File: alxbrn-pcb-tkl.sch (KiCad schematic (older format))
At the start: 24 parts, among them SW1 SW_Push, U1 ATmega32U4-AU, Y1 16MHz

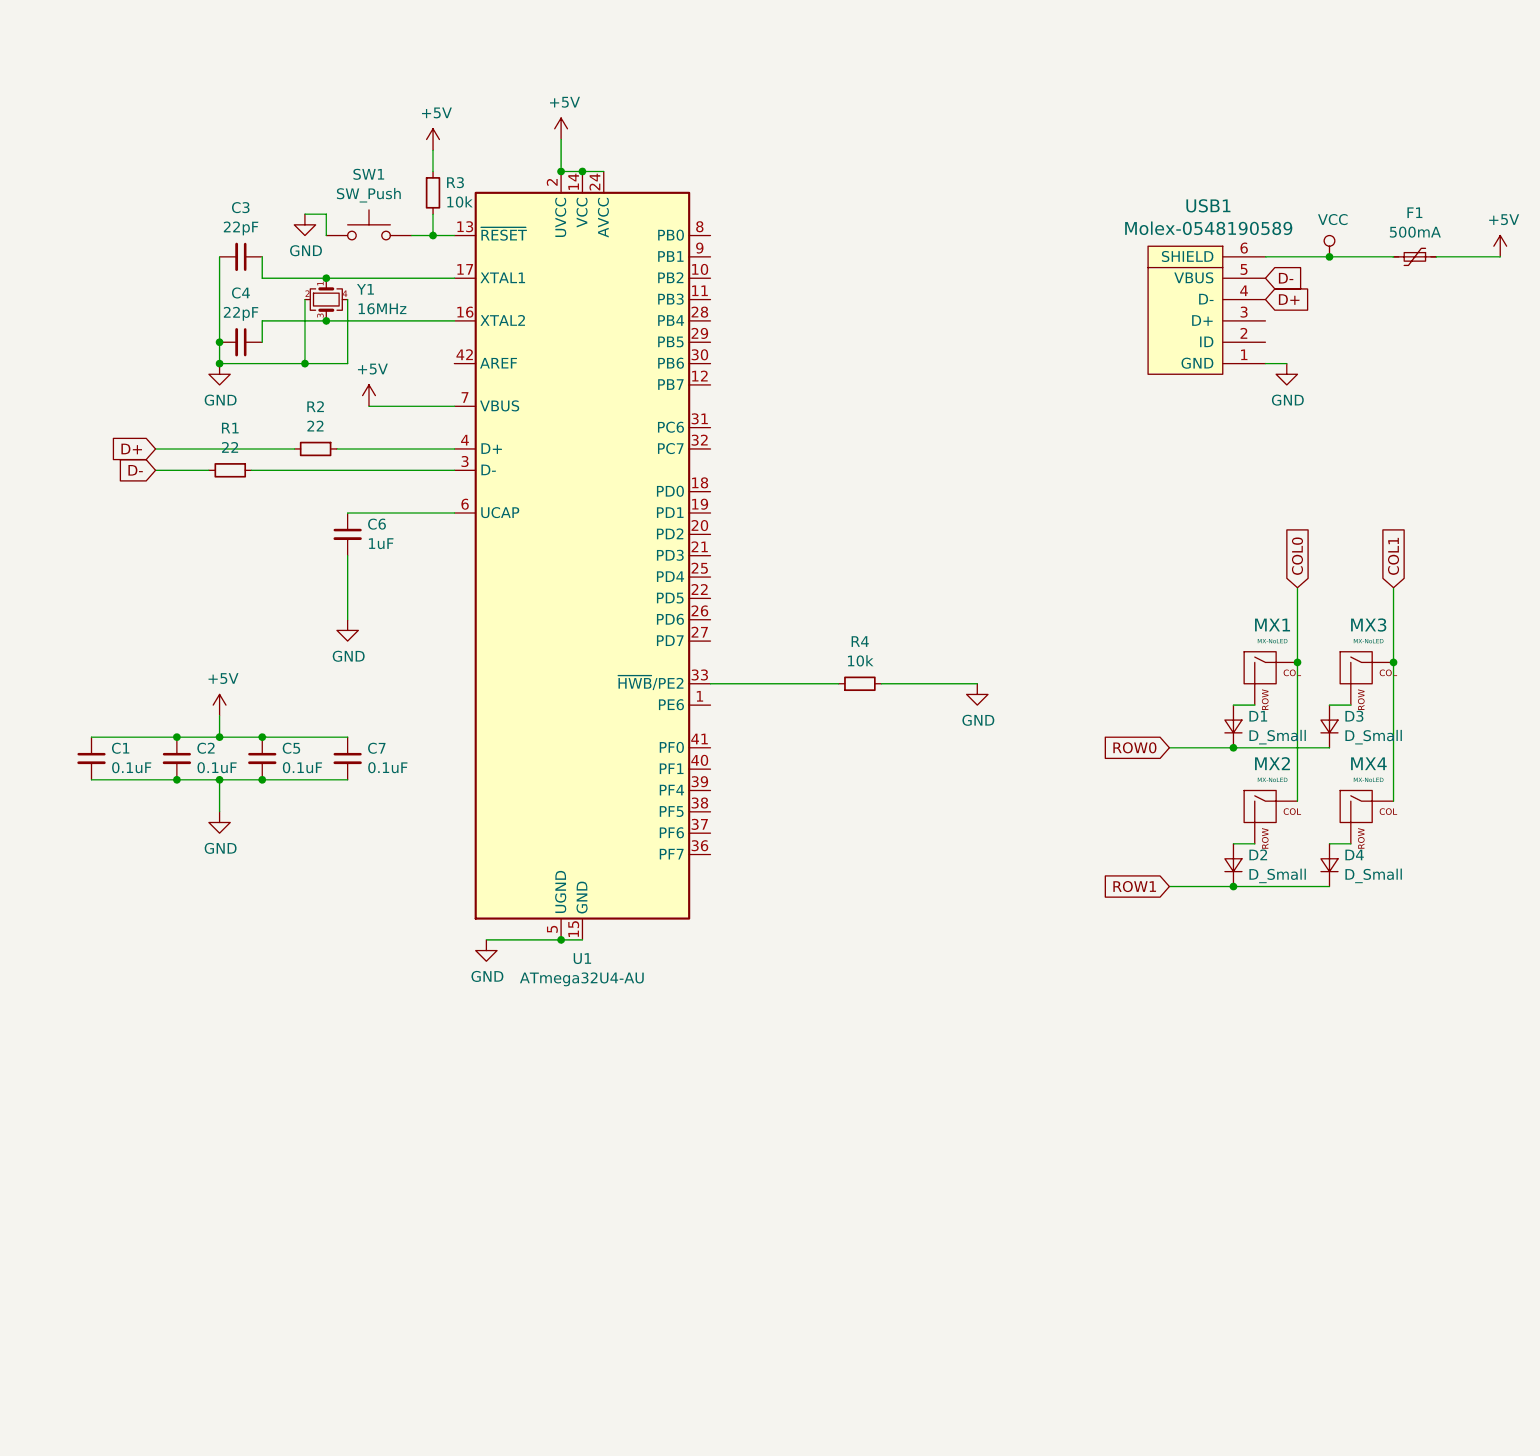
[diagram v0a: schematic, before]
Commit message: Schematic finished.
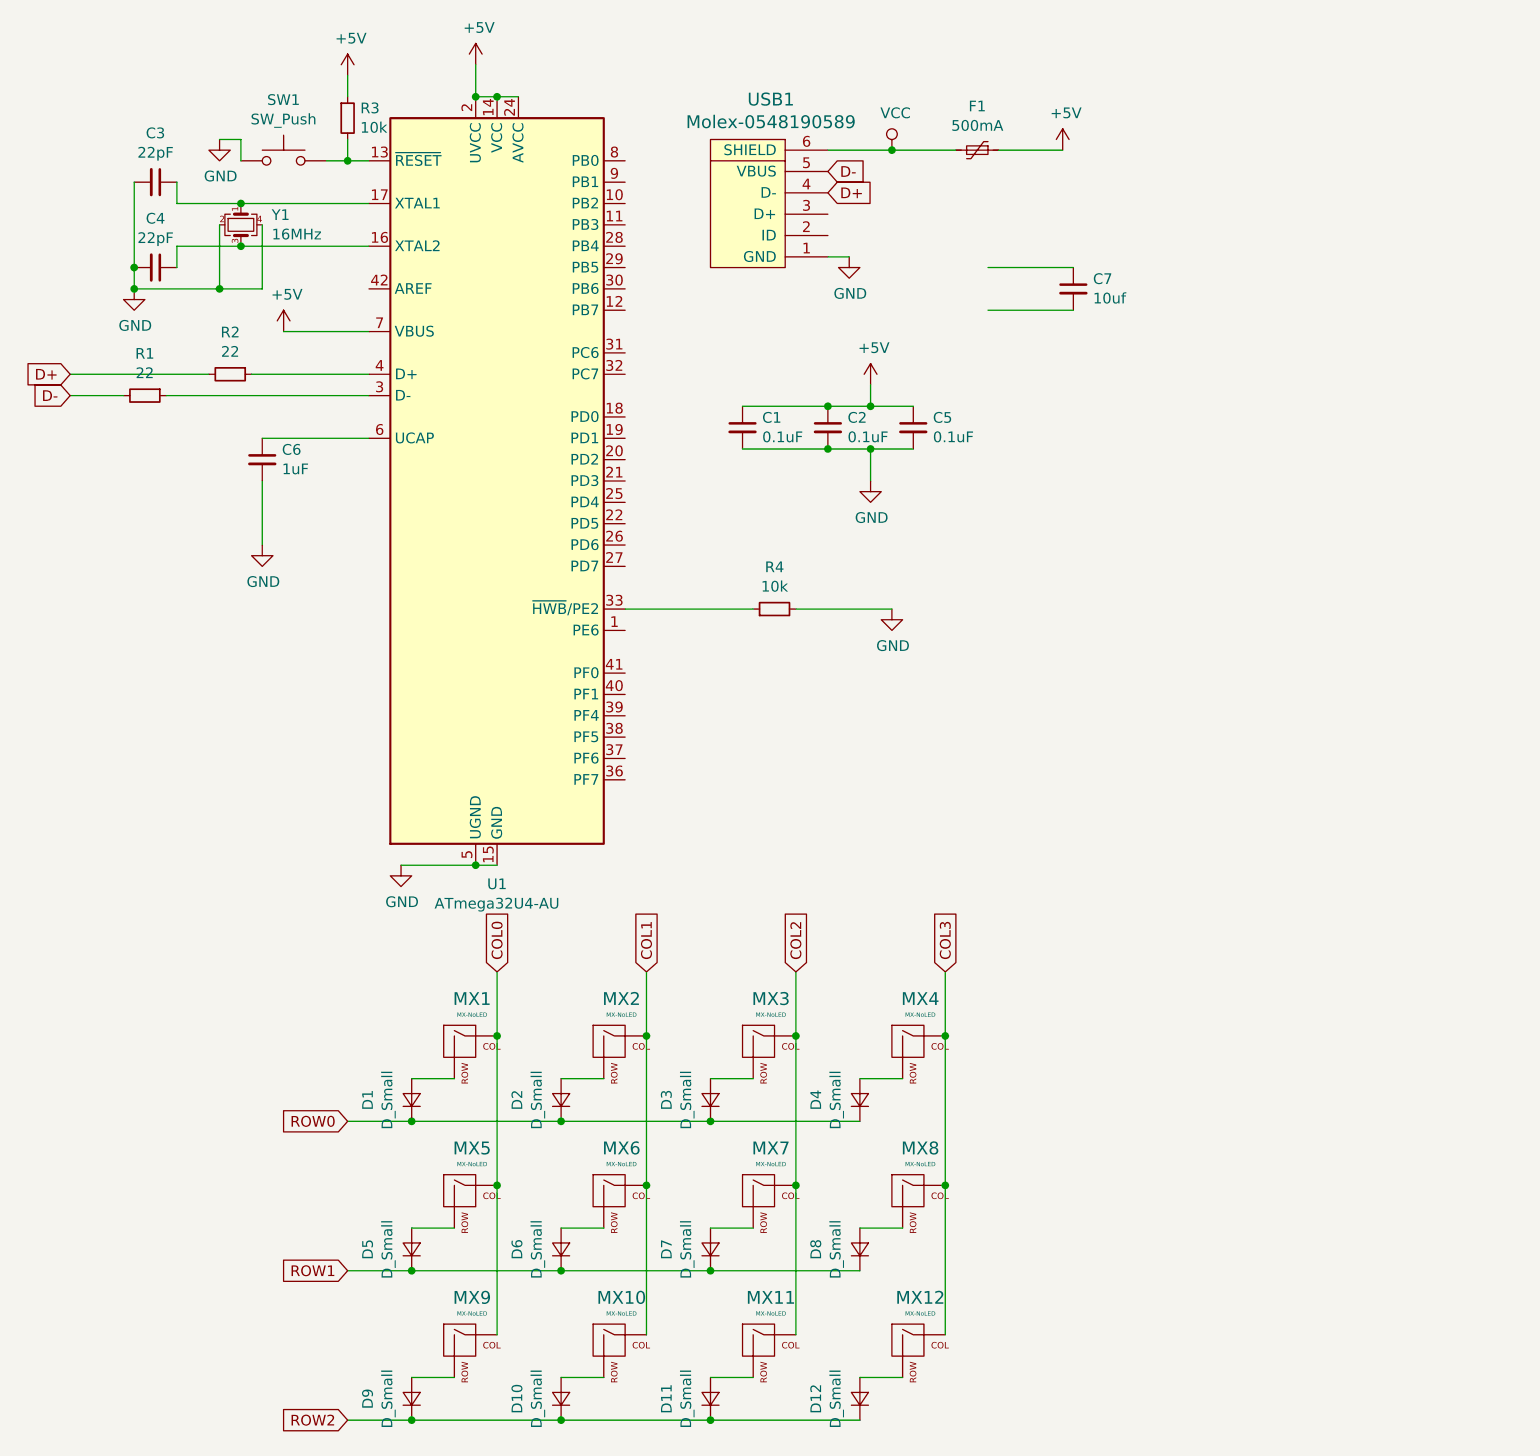
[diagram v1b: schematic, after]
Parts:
- added D10, D11, D12, D5, D6, D7, D8, D9: D_Small, Diode_SMD:D_SOD-123, symbol Device:D_Small
- added MX10, MX11, MX12, MX5, MX6, MX7, MX8, MX9: MX-NoLED, MX_Alps_Hybrid:MX-1U, symbol MX_Alps_Hybrid:MX-NoLED
- C7: value 0.1uF -> 10uf
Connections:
- net +5V: no longer C7.1
- net COL0: now also MX5.1 (COL), MX9.1 (COL); no longer MX2.1 (COL)
- net COL1: now also MX2.1 (COL), MX10.1 (COL), MX6.1 (COL); no longer MX3.1 (COL), MX4.1 (COL)
- net GND: no longer C7.2
- net ROW0: now also D2.1 (K), D4.1 (K)
- net ROW1: now also D5.1 (K), D6.1 (K), D7.1 (K), D8.1 (K); no longer D2.1 (K), D4.1 (K)
- new net: D5.2 (A), MX5.2 (ROW)
- new net: D6.2 (A), MX6.2 (ROW)
- new net: D7.2 (A), MX7.2 (ROW)
- new net: D8.2 (A), MX8.2 (ROW)
- new net: D9.2 (A), MX9.2 (ROW)
- new net: D10.2 (A), MX10.2 (ROW)
- new net: D11.2 (A), MX11.2 (ROW)
- new net: D12.2 (A), MX12.2 (ROW)
- new net COL2: MX11.1 (COL), MX3.1 (COL), MX7.1 (COL)
- new net COL3: MX12.1 (COL), MX4.1 (COL), MX8.1 (COL)
- new net ROW2: D10.1 (K), D11.1 (K), D12.1 (K), D9.1 (K)
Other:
- moved on the sheet: C1, C2, C3, C4, C5, C6, C7, F1, R1, R2, R3, R4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

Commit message: Possibly final commit.
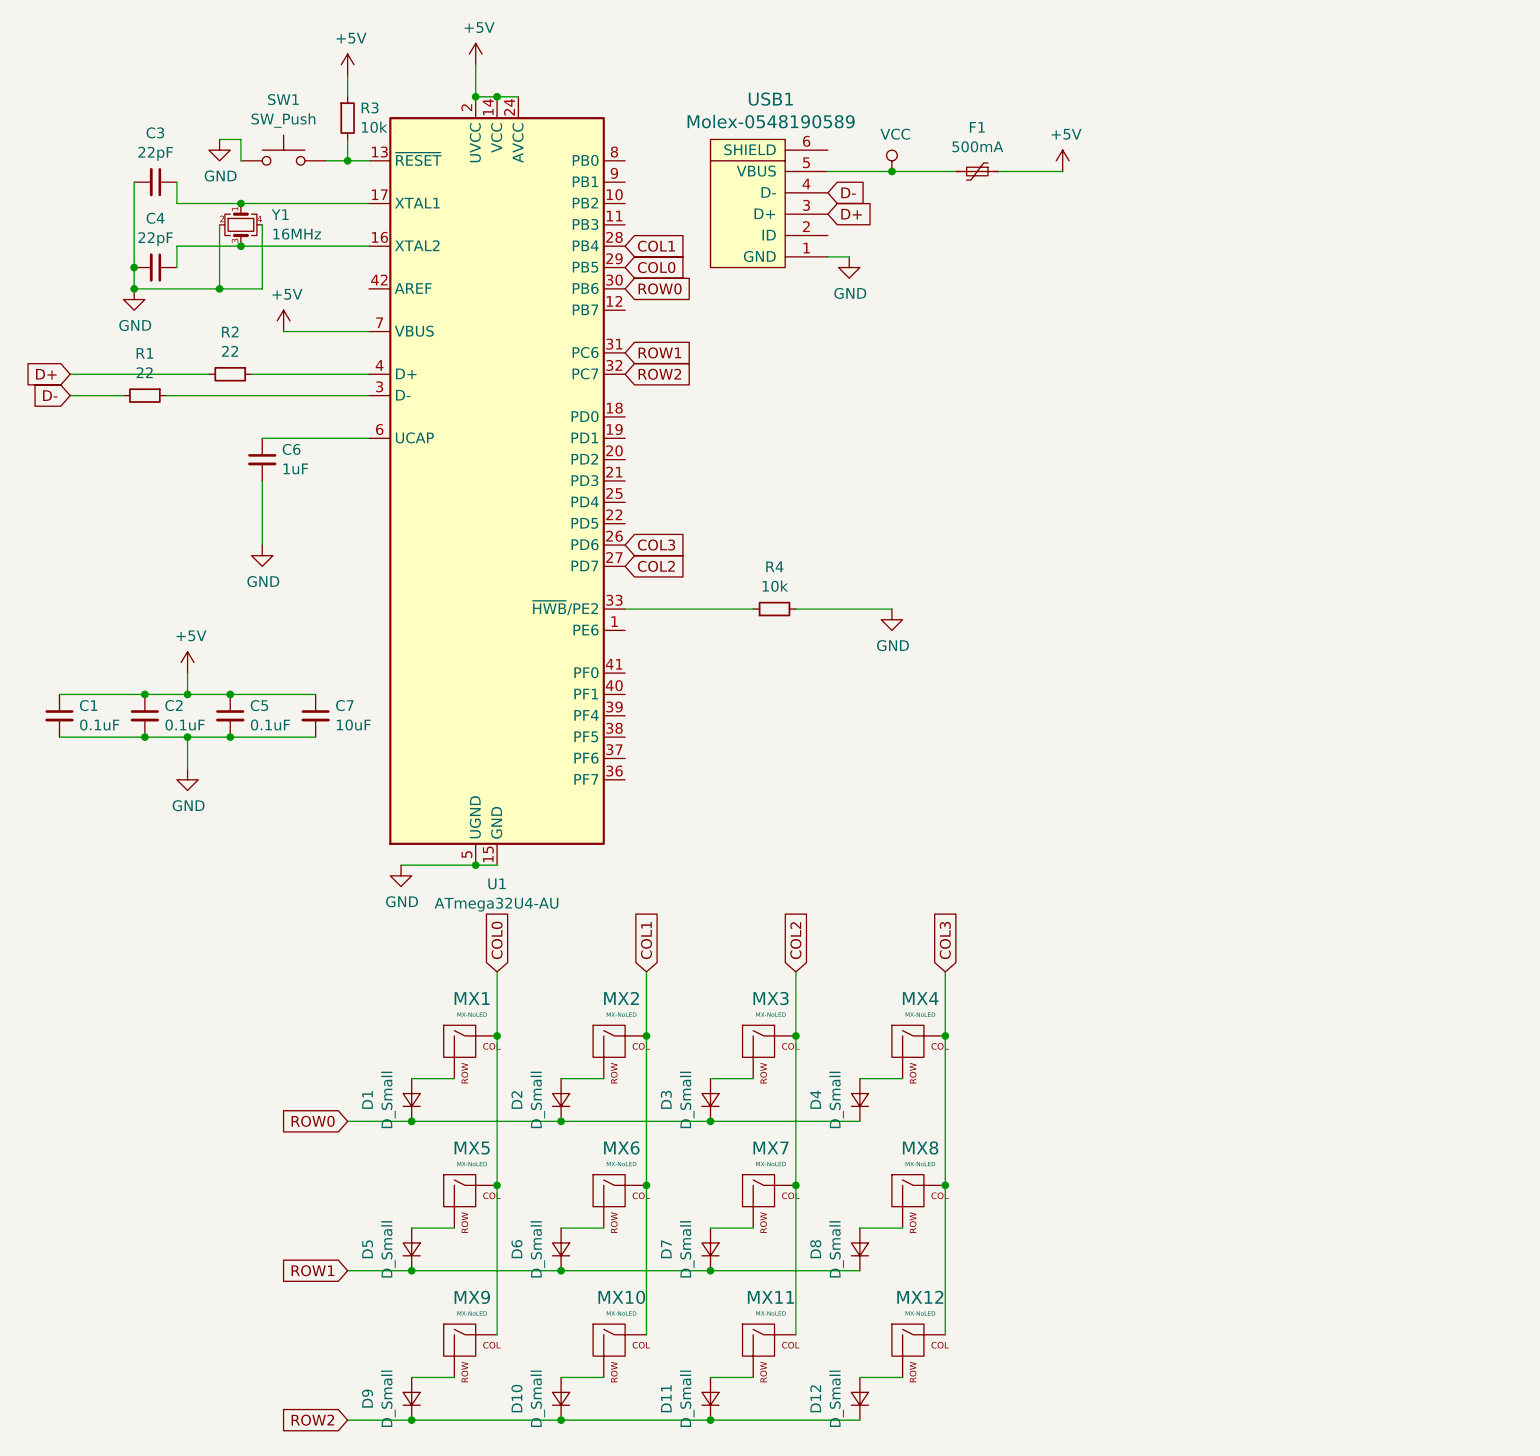
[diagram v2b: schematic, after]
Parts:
- C7: value 10uf -> 10uF
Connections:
- net +5V: now also C7.1
- net COL0: now also U1.29 (PB5)
- net COL1: now also U1.28 (PB4)
- net COL2: now also U1.27 (PD7)
- net COL3: now also U1.26 (PD6)
- net D+: now also USB1.3 (D+); no longer USB1.4 (D-)
- net D-: now also USB1.4 (D-); no longer USB1.5 (VBUS)
- net GND: now also C7.2
- net ROW0: now also U1.30 (PB6)
- net ROW1: now also U1.31 (PC6)
- net ROW2: now also U1.32 (PC7)
- net VCC: now also USB1.5 (VBUS); no longer USB1.6 (SHIELD)
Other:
- moved on the sheet: C1, C2, C5, F1
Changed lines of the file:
@@
 L power:+5V #PWR0105
 U 1 1 5E9B8DDC
-P 4600 2200
-F 0 "#PWR0105" H 4600 2050 50  0001 C CNN
-F 1 "+5V" H 4615 2373 50  0000 C CNN
-F 2 "" H 4600 2200 50  0001 C CNN
-F 3 "" H 4600 2200 50  0001 C CNN
-	1    4600 2200
+P 1400 3550
+F 0 "#PWR0105" H 1400 3400 50  0001 C CNN
+F 1 "+5V" H 1415 3723 50  0000 C CNN
+F 2 "" H 1400 3550 50  0001 C CNN
+F 3 "" H 1400 3550 50  0001 C CNN
+	1    1400 3550
 	1    0    0    -1
 $EndComp
@@
 L Device:C_Small C2
 U 1 1 5E9B9556
-P 4400 2400
-F 0 "C2" H 4492 2446 50  0000 L CNN
-F 1 "0.1uF" H 4492 2355 50  0000 L CNN
-F 2 "Capacitor_SMD:C_0805_2012Metric" H 4400 2400 50  0001 C CNN
-F 3 "~" H 4400 2400 50  0001 C CNN
-	1    4400 2400
+P 1200 3750
+F 0 "C2" H 1292 3796 50  0000 L CNN
+F 1 "0.1uF" H 1292 3705 50  0000 L CNN
+F 2 "Capacitor_SMD:C_0805_2012Metric" H 1200 3750 50  0001 C CNN
+F 3 "~" H 1200 3750 50  0001 C CNN
+	1    1200 3750
 	1    0    0    -1
 $EndComp
@@
 L Device:C_Small C5
 U 1 1 5E9BA173
-P 4800 2400
-F 0 "C5" H 4892 2446 50  0000 L CNN
-F 1 "0.1uF" H 4892 2355 50  0000 L CNN
-F 2 "Capacitor_SMD:C_0805_2012Metric" H 4800 2400 50  0001 C CNN
-F 3 "~" H 4800 2400 50  0001 C CNN
-	1    4800 2400
-	1    0    0    -1
-$EndComp
-$Comp
-L Device:C_Small C7
-U 1 1 5E9BA815
-P 5550 1750
-F 0 "C7" H 5642 1796 50  0000 L CNN
-F 1 "10uf" H 5642 1705 50  0000 L CNN
-F 2 "Capacitor_SMD:C_0805_2012Metric" H 5550 1750 50  0001 C CNN
-F 3 "~" H 5550 1750 50  0001 C CNN
-	1    5550 1750
+P 1600 3750
+F 0 "C5" H 1692 3796 50  0000 L CNN
+F 1 "0.1uF" H 1692 3705 50  0000 L CNN
+F 2 "Capacitor_SMD:C_0805_2012Metric" H 1600 3750 50  0001 C CNN
+F 3 "~" H 1600 3750 50  0001 C CNN
+	1    1600 3750
 	1    0    0    -1
 $EndComp
@@
 L Device:C_Small C1
 U 1 1 5E9BABB8
-P 4000 2400
-F 0 "C1" H 4092 2446 50  0000 L CNN
-F 1 "0.1uF" H 4092 2355 50  0000 L CNN
-F 2 "Capacitor_SMD:C_0805_2012Metric" H 4000 2400 50  0001 C CNN
-F 3 "~" H 4000 2400 50  0001 C CNN
-	1    4000 2400
-	1    0    0    -1
-$EndComp
-Wire Wire Line
-	4000 2500 4400 2500
-Connection ~ 4400 2500
-Wire Wire Line
-	5150 1850 5550 1850
-Wire Wire Line
-	5550 1650 5150 1650
-Wire Wire Line
-	4400 2300 4000 2300
-Connection ~ 4400 2300
+P 800 3750
+F 0 "C1" H 892 3796 50  0000 L CNN
+F 1 "0.1uF" H 892 3705 50  0000 L CNN
+F 2 "Capacitor_SMD:C_0805_2012Metric" H 800 3750 50  0001 C CNN
+F 3 "~" H 800 3750 50  0001 C CNN
+	1    800  3750
+	1    0    0    -1
+$EndComp
+Wire Wire Line
+	800  3850 1200 3850
+Connection ~ 1200 3850
+Wire Wire Line
+	1200 3650 800  3650
+Connection ~ 1200 3650
 $Comp
 L power:GND #PWR0106
 U 1 1 5E9B8886
-P 4600 2650
-F 0 "#PWR0106" H 4600 2400 50  0001 C CNN
-F 1 "GND" H 4605 2477 50  0000 C CNN
-F 2 "" H 4600 2650 50  0001 C CNN
-F 3 "" H 4600 2650 50  0001 C CNN
-	1    4600 2650
-	1    0    0    -1
-$EndComp
-Wire Wire Line
-	4400 2500 4600 2500
-Wire Wire Line
-	4400 2300 4600 2300
-Wire Wire Line
-	4600 2300 4600 2200
-Connection ~ 4600 2300
-Wire Wire Line
-	4600 2300 4800 2300
-Wire Wire Line
-	4600 2500 4600 2650
-Connection ~ 4600 2500
-Wire Wire Line
-	4600 2500 4800 2500
+P 1400 4000
+F 0 "#PWR0106" H 1400 3750 50  0001 C CNN
+F 1 "GND" H 1405 3827 50  0000 C CNN
+F 2 "" H 1400 4000 50  0001 C CNN
+F 3 "" H 1400 4000 50  0001 C CNN
+	1    1400 4000
+	1    0    0    -1
+$EndComp
+Wire Wire Line
+	1200 3850 1400 3850
+Wire Wire Line
+	1200 3650 1400 3650
+Wire Wire Line
+	1400 3650 1400 3550
+Connection ~ 1400 3650
+Wire Wire Line
+	1400 3650 1600 3650
+Wire Wire Line
+	1400 3850 1400 4000
+Connection ~ 1400 3850
+Wire Wire Line
+	1400 3850 1600 3850
 $Comp
 L power:+5V #PWR0107
@@
 L Device:Polyfuse_Small F1
 U 1 1 5E9E83C5
-P 5100 1100
-F 0 "F1" V 4895 1100 50  0000 C CNN
-F 1 "500mA" V 4986 1100 50  0000 C CNN
-F 2 "Fuse:Fuse_1206_3216Metric" H 5150 900 50  0001 L CNN
-F 3 "~" H 5100 1100 50  0001 C CNN
-	1    5100 1100
+P 5100 1200
+F 0 "F1" V 4895 1200 50  0000 C CNN
+F 1 "500mA" V 4986 1200 50  0000 C CNN
+F 2 "Fuse:Fuse_1206_3216Metric" H 5150 1000 50  0001 L CNN
+F 3 "~" H 5100 1200 50  0001 C CNN
+	1    5100 1200
 	0    1    1    0
 $EndComp
@@
 L power:+5V #PWR0111
 U 1 1 5E9E92BC
-P 5500 1100
-F 0 "#PWR0111" H 5500 950 50  0001 C CNN
-F 1 "+5V" H 5515 1273 50  0000 C CNN
-F 2 "" H 5500 1100 50  0001 C CNN
-F 3 "" H 5500 1100 50  0001 C CNN
-	1    5500 1100
+P 5500 1200
+F 0 "#PWR0111" H 5500 1050 50  0001 C CNN
+F 1 "+5V" H 5515 1373 50  0000 C CNN
+F 2 "" H 5500 1200 50  0001 C CNN
+F 3 "" H 5500 1200 50  0001 C CNN
+	1    5500 1200
 	1    0    0    -1
 $EndComp
@@
 L power:VCC #PWR0112
 U 1 1 5E9E9979
-P 4700 1100
-F 0 "#PWR0112" H 4700 950 50  0001 C CNN
-F 1 "VCC" H 4717 1273 50  0000 C CNN
-F 2 "" H 4700 1100 50  0001 C CNN
-F 3 "" H 4700 1100 50  0001 C CNN
-	1    4700 1100
-	1    0    0    -1
-$EndComp
-Wire Wire Line
-	4400 1100 4700 1100
-Wire Wire Line
-	4700 1100 5000 1100
-Connection ~ 4700 1100
-Wire Wire Line
-	5200 1100 5500 1100
-Text GLabel 4400 1200 2    50   Input ~ 0
+P 4700 1200
+F 0 "#PWR0112" H 4700 1050 50  0001 C CNN
+F 1 "VCC" H 4717 1373 50  0000 C CNN
+F 2 "" H 4700 1200 50  0001 C CNN
+F 3 "" H 4700 1200 50  0001 C CNN
+	1    4700 1200
+	1    0    0    -1
+$EndComp
+Wire Wire Line
+	4400 1200 4700 1200
+Wire Wire Line
+	4700 1200 5000 1200
+Connection ~ 4700 1200
+Wire Wire Line
+	5200 1200 5500 1200
+Text GLabel 4400 1300 2    50   Input ~ 0
 D-
-Text GLabel 4400 1300 2    50   Input ~ 0
+Text GLabel 4400 1400 2    50   Input ~ 0
 D+
 $Comp
@@
 Text GLabel 2150 7050 0    50   Input ~ 0
 ROW2
+$Comp
+L Device:C_Small C7
+U 1 1 5EAD1072
+P 2000 3750
+F 0 "C7" H 2092 3796 50  0000 L CNN
+F 1 "10uF" H 2092 3705 50  0000 L CNN
+F 2 "Capacitor_SMD:C_0805_2012Metric" H 2000 3750 50  0001 C CNN
+F 3 "~" H 2000 3750 50  0001 C CNN
+	1    2000 3750
+	1    0    0    -1
+$EndComp
+Wire Wire Line
+	1600 3650 2000 3650
+Connection ~ 1600 3650
+Wire Wire Line
+	1600 3850 2000 3850
+Connection ~ 1600 3850
+Text GLabel 3450 2950 2    50   Input ~ 0
+COL3
+Text GLabel 3450 3050 2    50   Input ~ 0
+COL2
+Text GLabel 3450 1550 2    50   Input ~ 0
+COL1
+Text GLabel 3450 1650 2    50   Input ~ 0
+COL0
+Text GLabel 3450 1750 2    50   Input ~ 0
+ROW0
+Text GLabel 3450 2050 2    50   Input ~ 0
+ROW1
+Text GLabel 3450 2150 2    50   Input ~ 0
+ROW2
 $EndSCHEMATC
